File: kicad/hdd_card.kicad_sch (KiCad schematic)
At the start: 11 parts, among them J1 POISK, U1 74LS245, U2 28C256, U3 74LS38, U4 74LS32, U5 74LS74

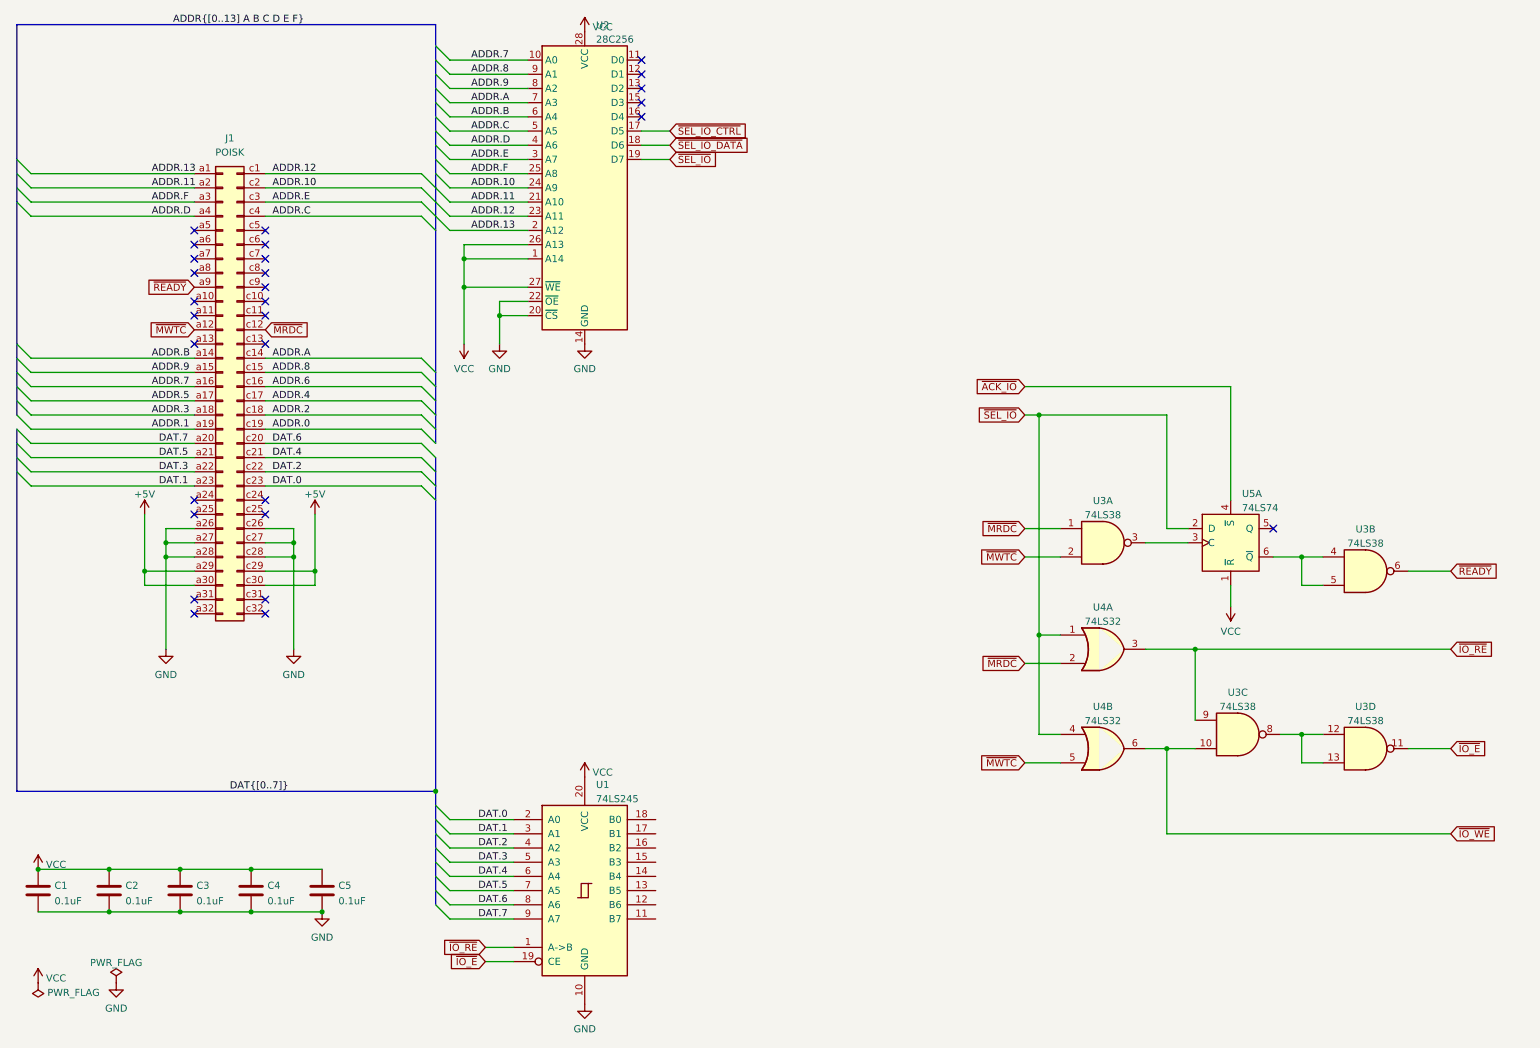
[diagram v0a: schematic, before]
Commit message: Schematics
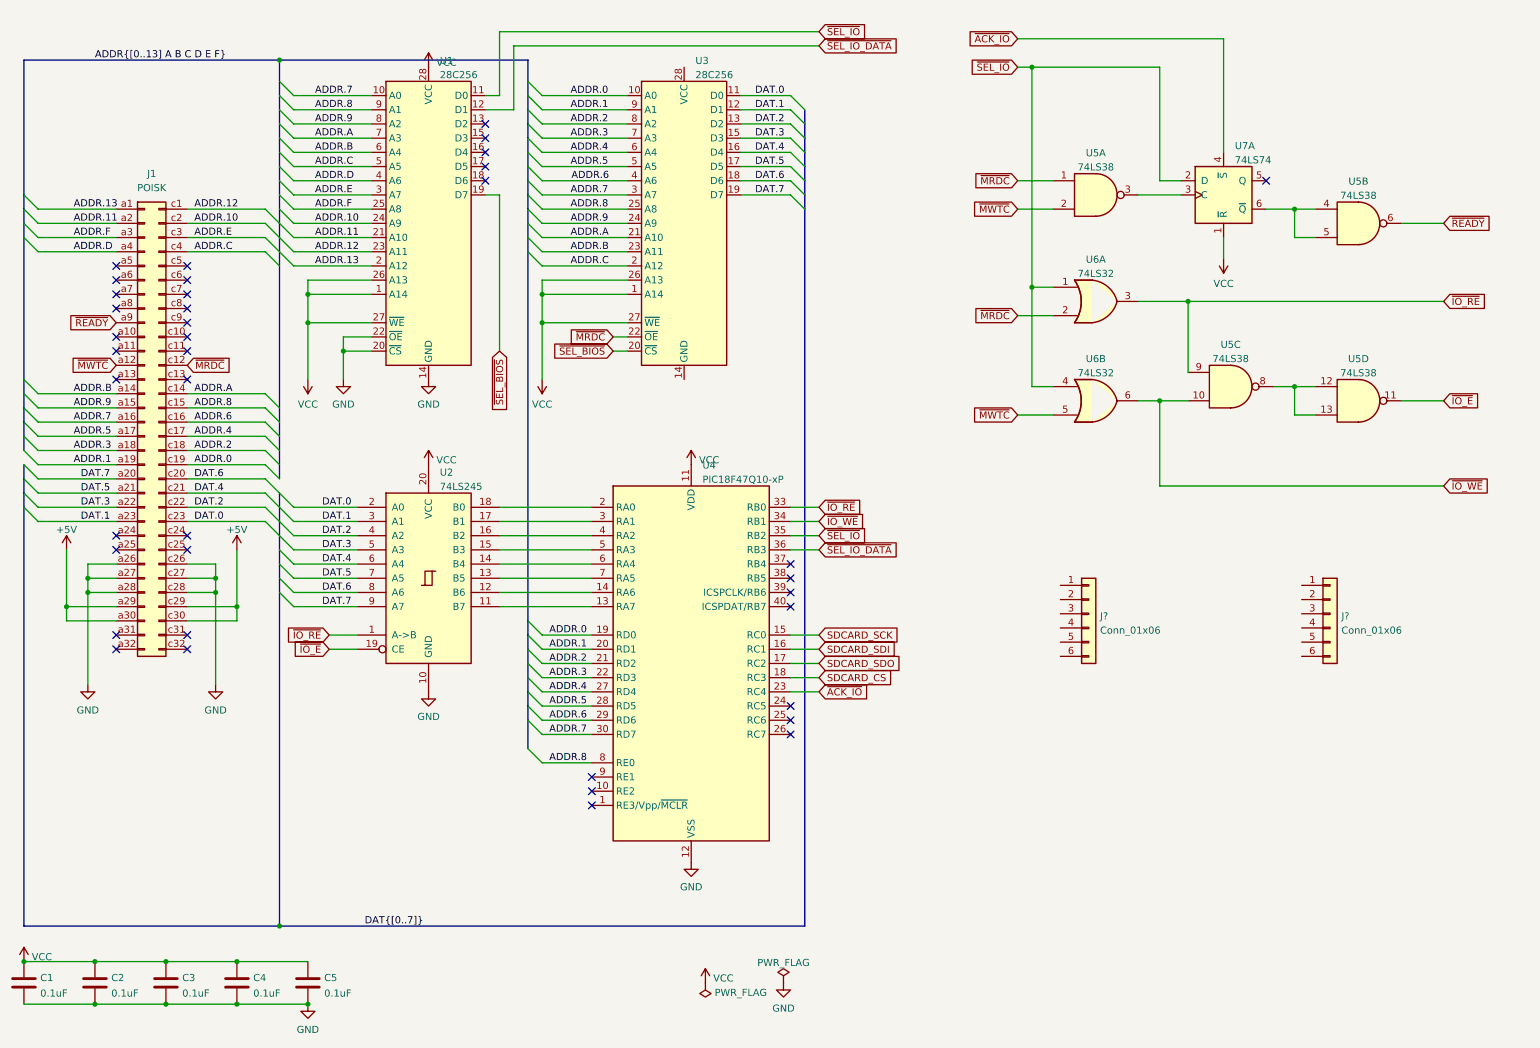
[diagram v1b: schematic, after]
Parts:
- added J? (x2): Conn_01x06, symbol Connector_Generic:Conn_01x06
- added U3: 28C256, symbol Memory_EEPROM:28C256
- added U4: PIC18F47Q10-xP, Package_DIP:DIP-40_W15.24mm, symbol MCU_Microchip_PIC18:PIC18F47Q10-xP
- renumbered U2 to U1, U1 to U2, U3 to U5, U4 to U6, U5 to U7
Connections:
- net ADDR.0: now also U3.10 (A0), U4.19 (RD0)
- net ADDR.1: now also U3.9 (A1), U4.20 (RD1)
- net ADDR.2: now also U3.8 (A2), U4.21 (RD2)
- net ADDR.3: now also U3.7 (A3), U4.22 (RD3)
- net ADDR.4: now also U3.6 (A4), U4.27 (RD4)
- net ADDR.5: now also U3.5 (A5), U4.28 (RD5)
- net ADDR.6: now also U3.4 (A6), U4.29 (RD6)
- net ADDR.7: now also U3.3 (A7), U4.30 (RD7)
- net ADDR.8: now also U3.25 (A8), U4.8 (RE0)
- net ADDR.9: now also U3.24 (A9)
- net ADDR.A: now also U3.21 (A10)
- net ADDR.B: now also U3.23 (A11)
- net ADDR.C: now also U3.2 (A12)
- net DAT.0: now also U3.11 (D0)
- net DAT.1: now also U3.12 (D1)
- net DAT.2: now also U3.13 (D2)
- net DAT.3: now also U3.15 (D3)
- net DAT.4: now also U3.16 (D4)
- net DAT.5: now also U3.17 (D5)
- net DAT.6: now also U3.18 (D6)
- net DAT.7: now also U3.19 (D7)
- net GND: now also U4.12 (VSS), U4.31 (VSS)
- net VCC: now also U3.1 (A14), U3.26 (A13), U3.27 (~{WE}), U4.11 (VDD), U4.32 (VDD)
- net ~{ACK_IO}: now also U4.23 (RC4)
- net ~{IO_RE}: now also U4.33 (RB0)
- net ~{IO_WE}: now also U4.34 (RB1)
- net ~{MRDC}: now also U3.22 (~{OE})
- net ~{SEL_IO_DATA}: now also U1.12 (D1), U4.36 (RB3); no longer U1.18 (D6)
- net ~{SEL_IO}: now also U1.11 (D0), U4.35 (RB2); no longer U1.19 (D7)
- net at U2.11 (B7): now also U4.13 (RA7)
- net at U2.12 (B6): now also U4.14 (RA6)
- net at U2.13 (B5): now also U4.7 (RA5)
- net at U2.14 (B4): now also U4.6 (RA4)
- net at U2.15 (B3): now also U4.5 (RA3)
- net at U2.16 (B2): now also U4.4 (RA2)
- net at U2.17 (B1): now also U4.3 (RA1)
- net at U2.18 (B0): now also U4.2 (RA0)
- net ~{SEL_IO_CTRL}: no longer names the net of U1.17 (D5)
- new net SDCARD_CS: U4.18 (RC3)
- new net SDCARD_SCK: U4.15 (RC0)
- new net SDCARD_SDI: U4.16 (RC1)
- new net SDCARD_SDO: U4.17 (RC2)
- new net ~{SEL_BIOS}: U1.19 (D7), U3.20 (~{CS})
- no-connect marks 29 -> 39
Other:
- moved on the sheet: C1, C2, C3, C4, C5, J1, U1, U2, U5A, U5B, U5C, U5D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

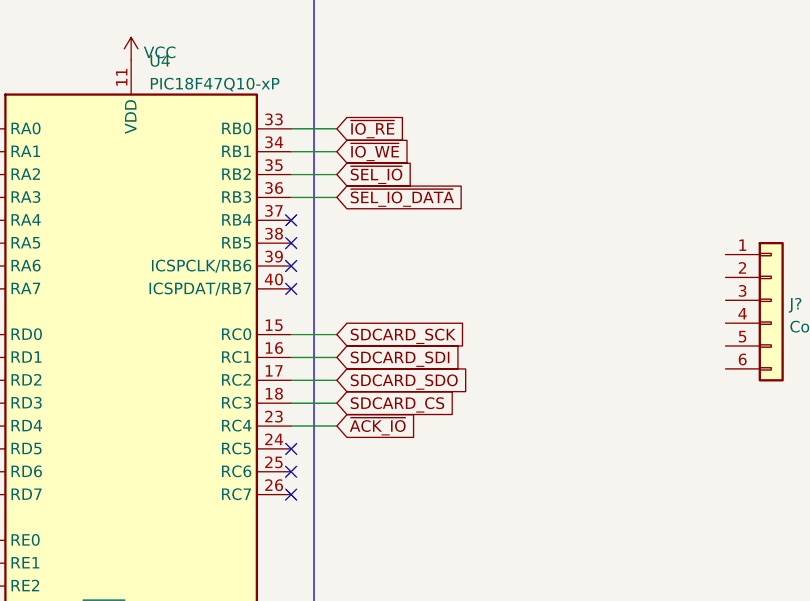
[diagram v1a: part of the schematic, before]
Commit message: Adjust schematic
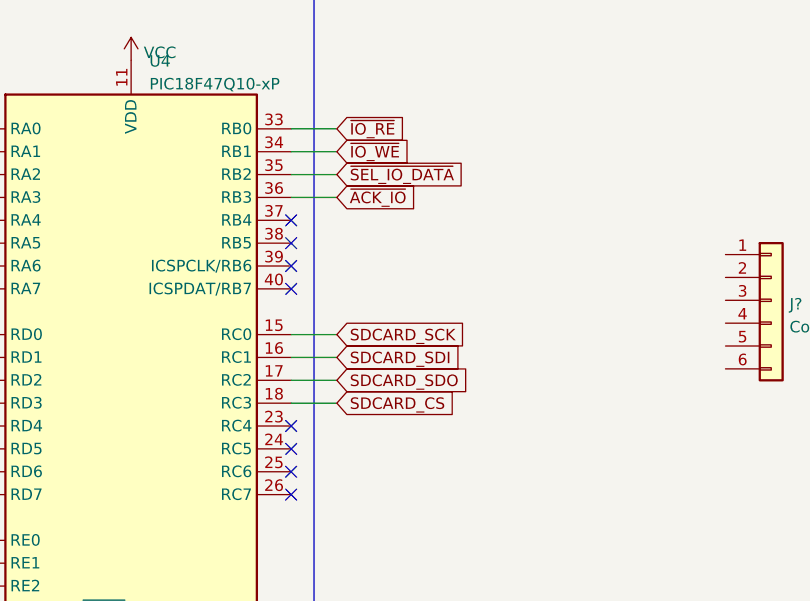
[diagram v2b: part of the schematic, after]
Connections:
- net ~{ACK_IO}: now also U4.36 (RB3); no longer U4.23 (RC4)
- net ~{SEL_IO_DATA}: now also U4.35 (RB2); no longer U4.36 (RB3)
- net ~{SEL_IO}: no longer U4.35 (RB2)
- no-connect marks 39 -> 40
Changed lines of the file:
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@@
   (no_connect (at 46.99 59.69))
   (no_connect (at 100.33 41.91))
+  (no_connect (at 154.94 135.89))
   (no_connect (at 154.94 113.03))
   (no_connect (at 154.94 140.97))
@@
     (stroke (width 0) (type default) (color 0 0 0 0))
   )
-  (wire (pts (xy 154.94 135.89) (xy 160.02 135.89))
+  (wire (pts (xy 154.94 110.49) (xy 160.02 110.49))
     (stroke (width 0) (type default) (color 0 0 0 0))
   )
@@
   )
   (bus (pts (xy 17.78 92.71) (xy 17.78 90.17))
-    (stroke (width 0) (type default) (color 0 0 0 0))
-  )
-  (wire (pts (xy 154.94 110.49) (xy 160.02 110.49))
     (stroke (width 0) (type default) (color 0 0 0 0))
   )
@@
     )
   )
-  (global_label "~{SEL_IO_DATA}" (shape input) (at 160.02 110.49 0) (fields_autoplaced)
+  (global_label "~{SEL_IO_DATA}" (shape input) (at 160.02 107.95 0) (fields_autoplaced)
     (effects (font (size 1.27 1.27)) (justify left))
-    (property "Intersheet References" "${INTERSHEET_REFS}" (id 0) (at 174.105 110.4106 0)
+    (property "Intersheet References" "${INTERSHEET_REFS}" (id 0) (at 174.105 107.8706 0)
       (effects (font (size 1.27 1.27)) (justify left) hide)
     )
@@
     )
   )
-  (global_label "~{ACK_IO}" (shape input) (at 160.02 135.89 0) (fields_autoplaced)
+  (global_label "~{ACK_IO}" (shape input) (at 160.02 110.49 0) (fields_autoplaced)
     (effects (font (size 1.27 1.27)) (justify left))
-    (property "Intersheet References" "${INTERSHEET_REFS}" (id 0) (at 168.9645 135.9694 0)
+    (property "Intersheet References" "${INTERSHEET_REFS}" (id 0) (at 168.9645 110.5694 0)
       (effects (font (size 1.27 1.27)) (justify left) hide)
     )
@@
       (effects (font (size 1.27 1.27)) (justify left) hide)
     )
-  )
-  (global_label "~{SEL_IO}" (shape input) (at 160.02 107.95 0) (fields_autoplaced)
-    (effects (font (size 1.27 1.27)) (justify left))
-    (property "Intersheet References" "${INTERSHEET_REFS}" (id 0) (at 168.7226 107.8706 0)
-      (effects (font (size 1.27 1.27)) (justify left) hide)
-    )
